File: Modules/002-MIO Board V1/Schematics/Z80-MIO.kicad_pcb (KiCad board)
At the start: 2 copper layers, 160 x 100.3 mm, 77 parts, among them J1 Conn_02x05_Odd_Even, J2 Conn_02x32_Row_Letter_First, J3 Conn_02x02_Top_Bottom, J4 Conn_02x06_Odd_Even, J5 Mini-DIN-6, J6 Mini-DIN-6, J7 Jumper_2_Bridged, J8 Conn_02x04_Odd_Even, J9 Conn_02x04_Odd_Even, Q1 BC548, U1 74HC688, U10 DS1307+, U11 74HC161, U12 Am9511A, U2 GAL16V8, U3 74HC245, U4 74HC245, U5 74HC245, U6 PIO-DIP-40, U7 74LS06, U8 PCF8584, U9 8048, Y1 32.768 kHz

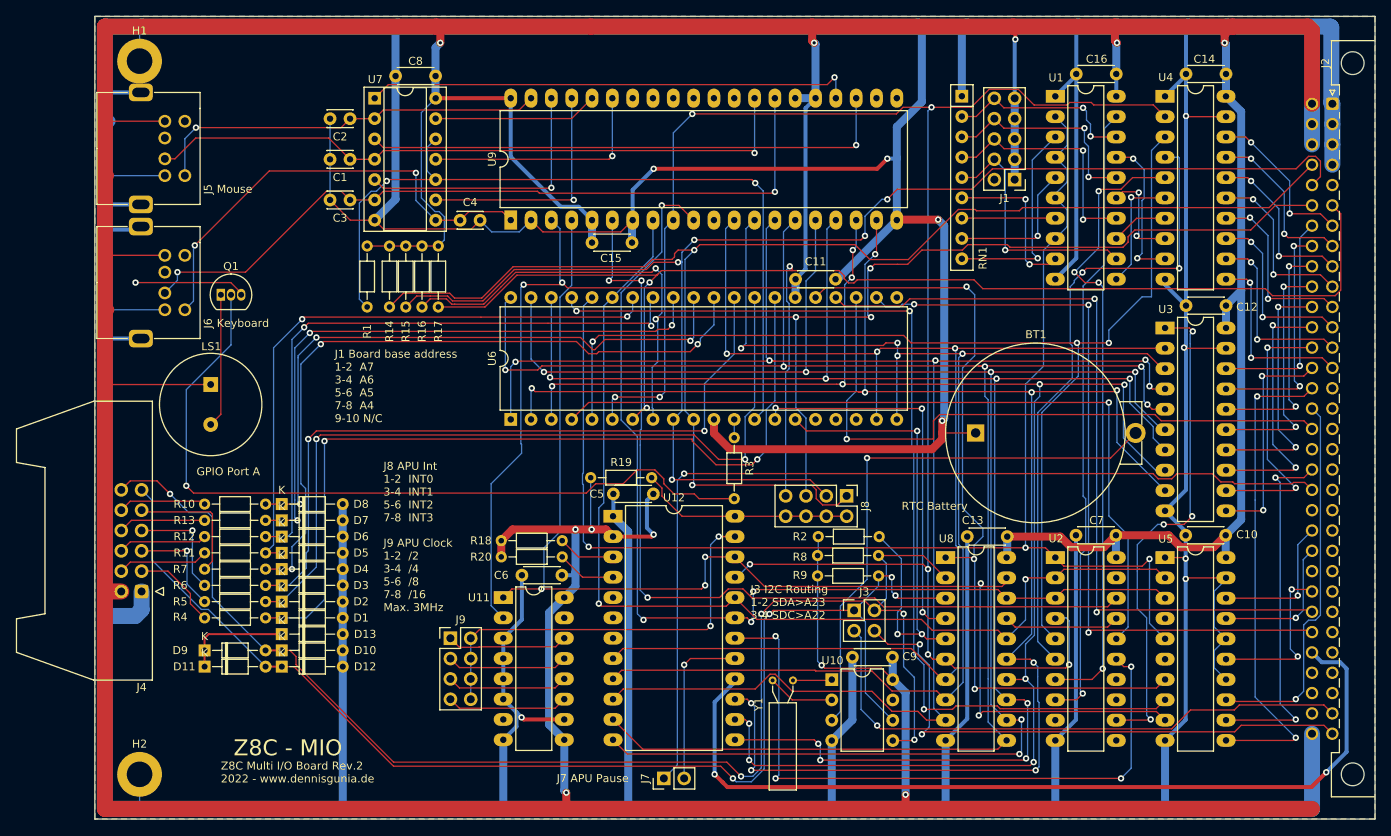
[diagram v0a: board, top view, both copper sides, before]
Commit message: multiple updates
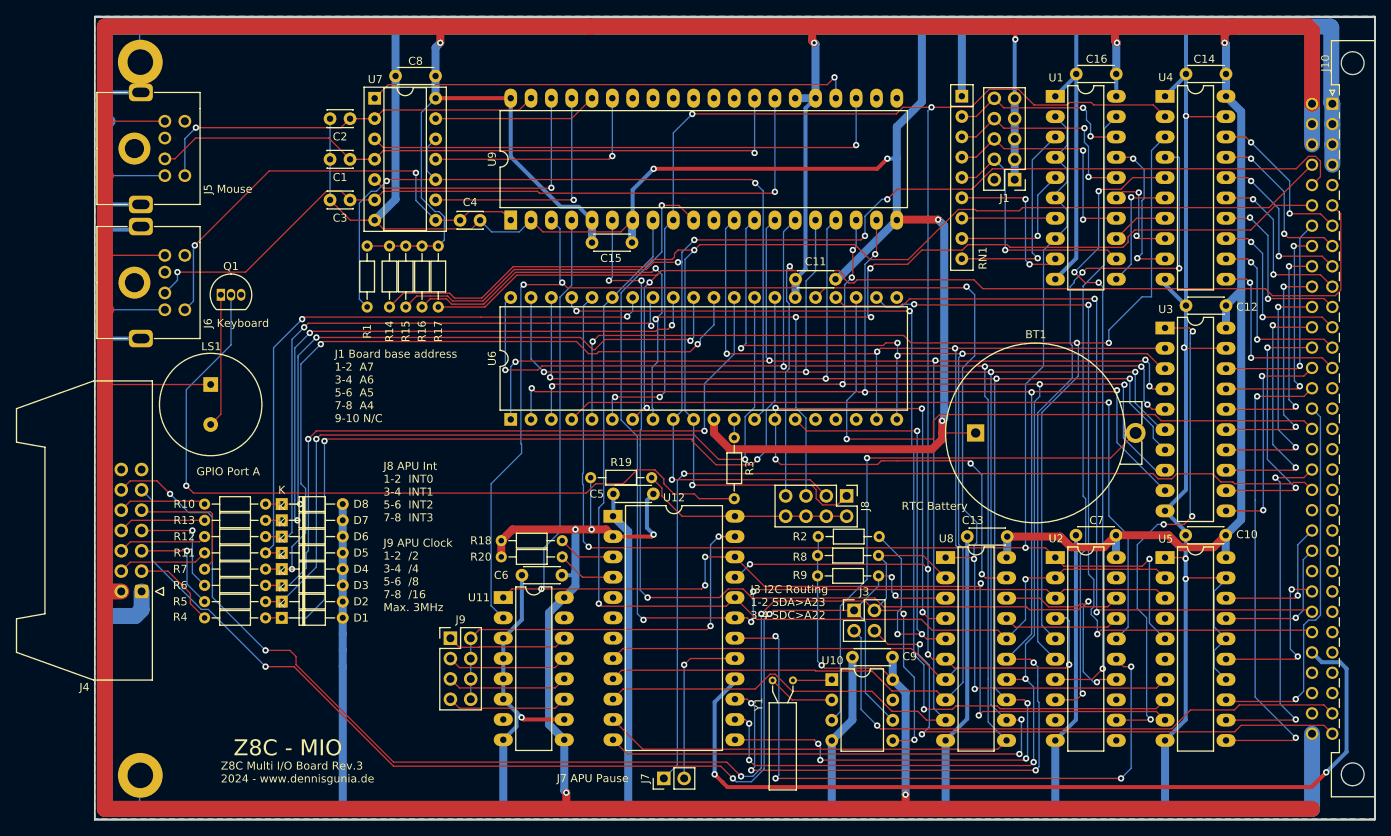
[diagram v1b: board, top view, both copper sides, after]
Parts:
- removed D10, D11, D12, D9: D, Diode_THT:D_DO-34_SOD68_P7.62mm_Horizontal
- removed D13: 5.1V, Diode_THT:D_DO-34_SOD68_P7.62mm_Horizontal
- removed H1, H2: MountingHole_Pad, MountingHole:MountingHole_3.2mm_M3_DIN965_Pad
- removed J2: Conn_02x32_Row_Letter_First, Connector_DIN:DIN41612_Q_2x32_Male_Horizontal_THT
- added J10: Z8C_Card, Dennis:Z8C Card, F.Cu at (199.4, 98.6)
- J4: value Conn_02x06_Odd_Even -> Conn_02x07_Odd_Even; footprint Connector_IDC:IDC-Header_2x06_P2.54mm_Latch_Horizontal -> Connector_IDC:IDC-Header_2x07_P2.54mm_Latch_Horizontal
- J5, J6: footprint w_conn_av:PS2 -> Dennis:PS2
- R8, R9: value R -> 4k7
- U3: value 74HC245 -> 74HC2T45
- U7: value 74LS06 -> 7406
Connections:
- net /CS_FPU renamed /~{CS_FPU}
- net /CS_IIC renamed /~{CS_IIC}
- net /CS_PS2 renamed /~{CS_PS2}
- net Net-(J9-Pad2) renamed /FPU_CLK
- net Net-(R1-Pad2) renamed /~{INT_KB}
- net Net-(R2-Pad2) renamed /~{INT_IIC}
- net Net-(R3-Pad1) renamed /SPK_DRV
- net Net-(U2-Pad16) renamed /~{CS_PIO}
- J3 pad 1: /I2C_SCL -> /A22/SCL
- J3 pad 2: /I2C_SDA -> /A23/SDA
- U2 pad 14: unconnected-(U2-Pad14) -> /~{IIC_WR}
- U2 pad 19: /BOARD_CS -> unconnected-(U2-IO1-Pad19)
- U6 pad 14: Net-(U6-Pad14) -> /~{RST_IIC}
- U8 pad 18: /~{#WR} -> /~{IIC_WR}
- U8 pad 19: /~{#RESET} -> /~{RST_IIC}
- U8 pad 4: Net-(U6-Pad14) -> +5V
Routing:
- net +5V: track 811.7 -> 860.2 mm, vias 11 -> 14
- net Net-(U6-Pad14): track 48.5 -> 0.00 mm, vias 3 -> 0
- net /~{RST_IIC}: track 0.00 -> 47.5 mm, vias 0 -> 3
- net /~{IIC_WR}: track 0.00 -> 24.9 mm, vias 0 -> 2
- net GND: track 1114.8 -> 1101.1 mm, vias 10 -> 9
- net Net-(D11-Pad1): track 13.4 -> 0.00 mm
- net /~{#RESET}: track 157.9 -> 154.2 mm
- net /#CLK_CPU: track 190.7 -> 190.0 mm
- net /I2C_SDA: vias 5 -> 6
- net /I2C_SCL: vias 4 -> 5
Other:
- board text added: "Z8C Multi I/O Board Rev.3 2024 - www.dennisgunia.de"
- board text removed: "Z8C Multi I/O Board Rev.2 2022 - www.dennisgunia.de"
